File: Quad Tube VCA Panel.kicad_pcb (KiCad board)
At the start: 2 copper layers, 162.6 x 128.5 mm, 0 parts

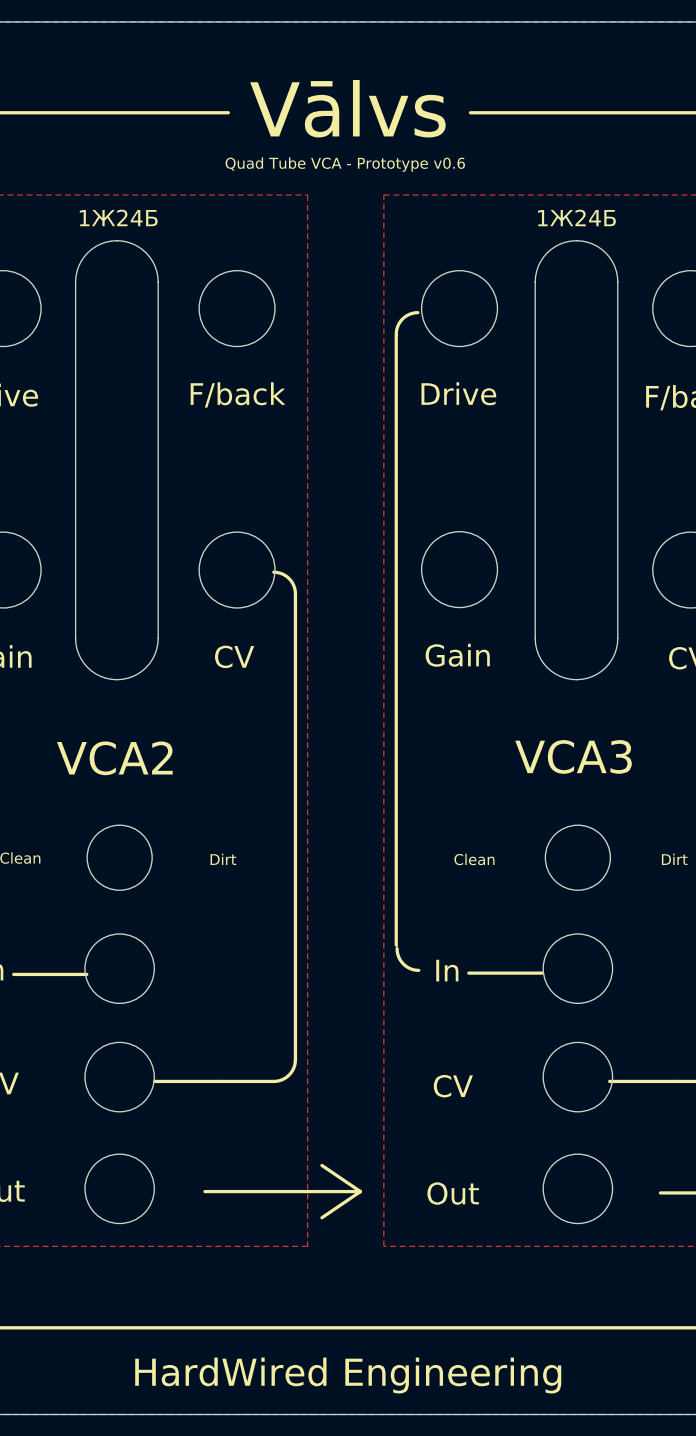
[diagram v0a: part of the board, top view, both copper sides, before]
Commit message: updates v0.6 gerbers
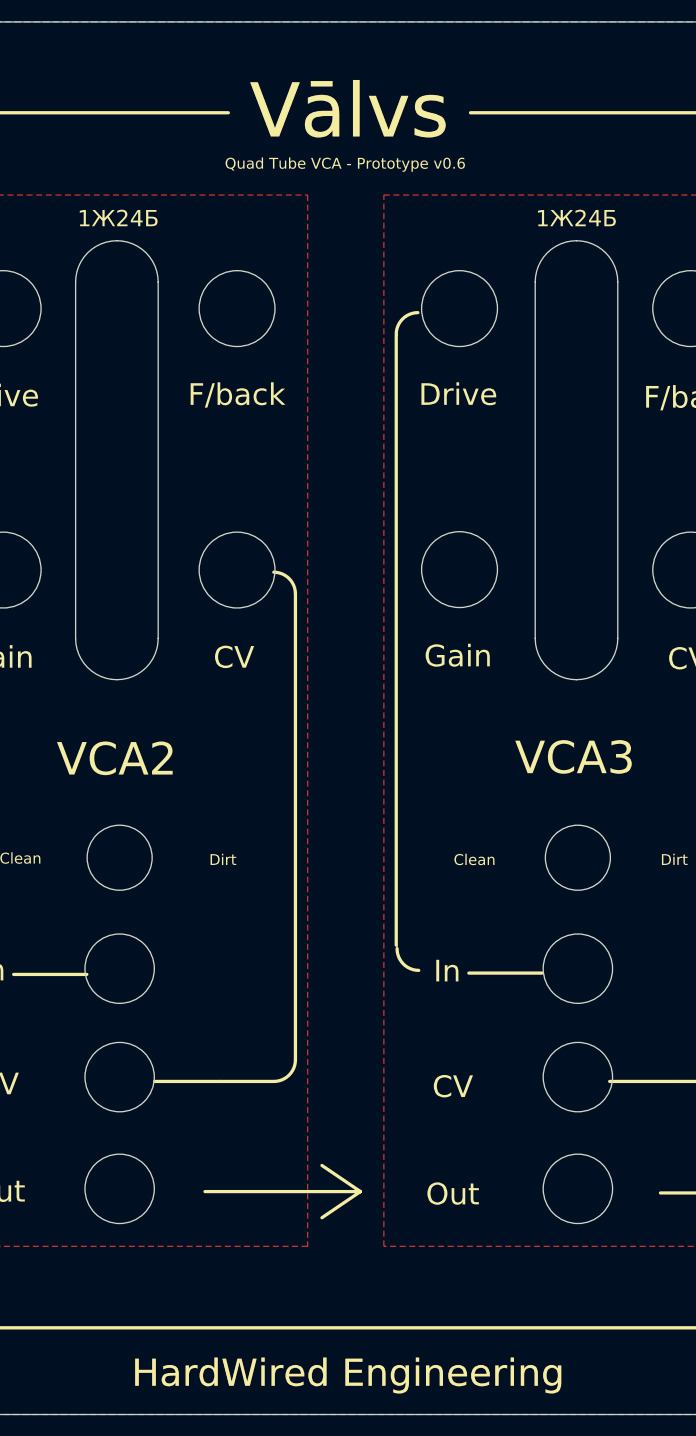
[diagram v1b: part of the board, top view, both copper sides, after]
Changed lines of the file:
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@@
   (general
     (thickness 1.6)
-    (drawings 175)
+    (drawings 177)
     (tracks 4)
     (zones 0)
@@
     (uvia_drill 0.1)
   )
+  (gr_text "HardWired Engineering" (at 88.011 185.42) (layer F.Cu)
+    (effects (font (size 2.5 2.5) (thickness 0.25)))
+  )
+  (gr_text Vālvs (at 88.138 68.961) (layer F.Cu)
+    (effects (font (size 5 5) (thickness 0.5)))
+  )
   (gr_text Drive (at 55.88 95.25) (layer F.SilkS)
